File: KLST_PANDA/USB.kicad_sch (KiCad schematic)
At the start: 11 parts, among them J16 DEVICE+CHARGE(UFP), J17 HOST(DFP)

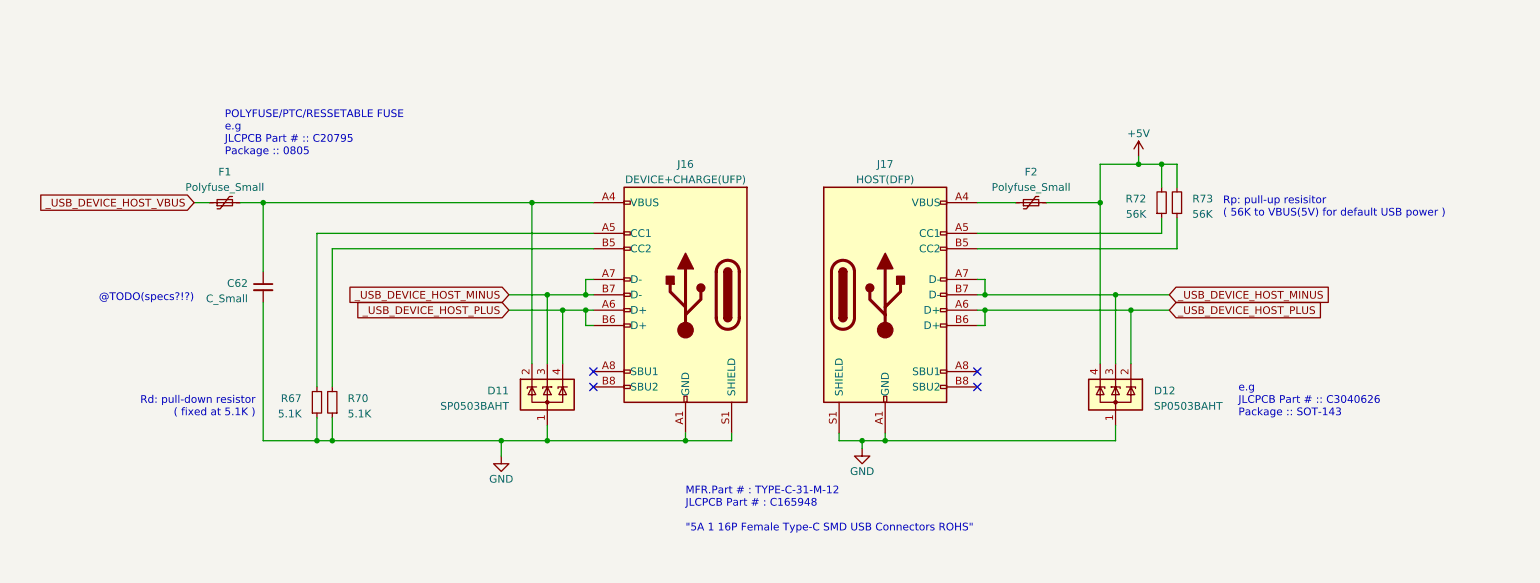
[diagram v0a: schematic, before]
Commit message: cleaned up main sheet
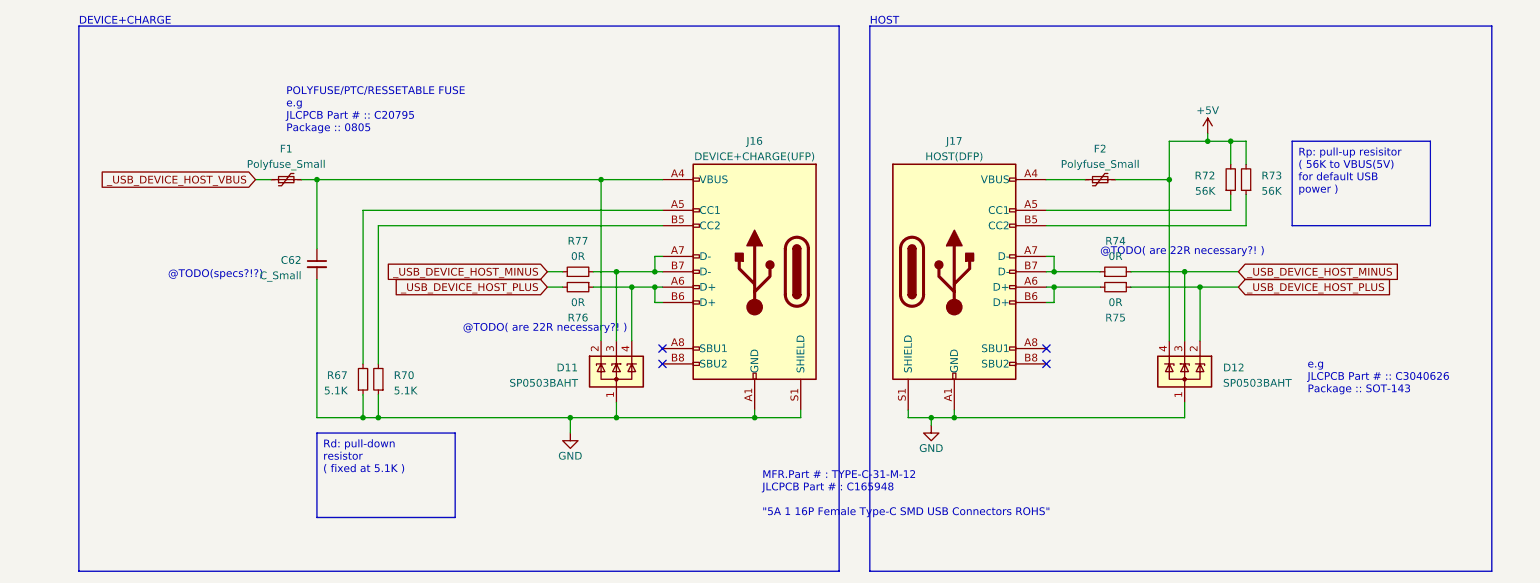
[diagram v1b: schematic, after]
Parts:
- added R74, R75, R76, R77: 0R, symbol Device:R_Small
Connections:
- net _USB_DEVICE_HOST_MINUS: now also R74.2, R77.1; no longer D11.3 (K), J16.A7 (D-), J16.B7 (D-), J17.A7 (D-), J17.B7 (D-)
- net _USB_DEVICE_HOST_PLUS: now also R75.1, R76.2; no longer D11.4 (K), J16.A6 (D+), J16.B6 (D+), J17.A6 (D+), J17.B6 (D+)
- new net: D11.4 (K), J16.A6 (D+), J16.B6 (D+), R76.1
- new net: J17.A6 (D+), J17.B6 (D+), R75.2
- new net: D11.3 (K), J16.A7 (D-), J16.B7 (D-), R77.2
- new net: J17.A7 (D-), J17.B7 (D-), R74.1
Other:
- note added: "@TODO( are 22R necessary?! )"
- note added: "DEVICE+CHARGE"
- note added: "HOST"
- note removed: "Rd: pull-down resistor ( fixed at 5.1K )"
- note removed: "Rp: pull-up resisitor ( 56K to VBUS(5V) for default USB power )"
- moved on the sheet: C62, D11, D12, F1, F2, J16, J17, R67, R70, R72, R73
